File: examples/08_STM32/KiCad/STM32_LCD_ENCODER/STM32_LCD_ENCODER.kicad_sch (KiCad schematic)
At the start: 18 parts, among them J1 Audio In, SW1 ENCODER, U1 STM32F103C6Tx, U2 LCD16X2, X1 ACO-32.768MHz

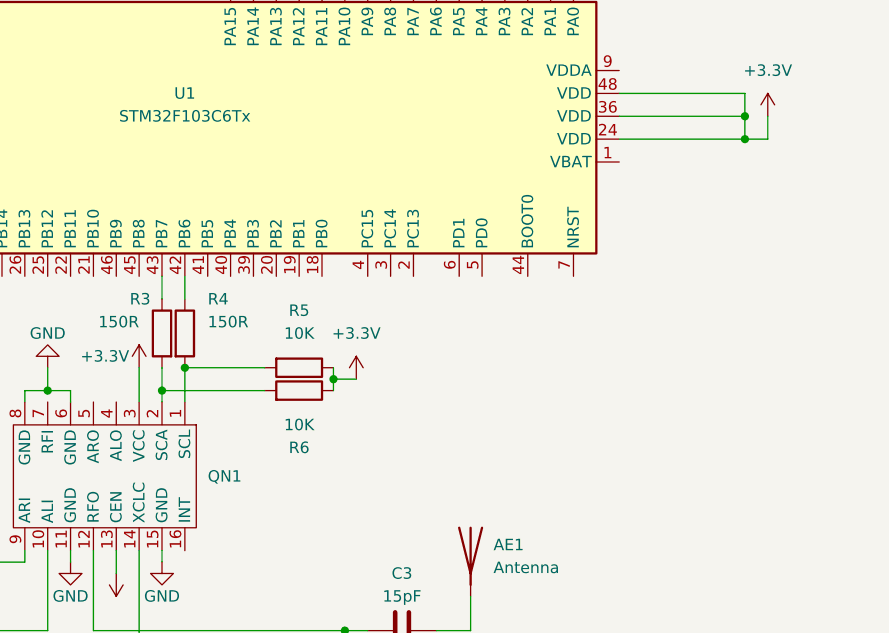
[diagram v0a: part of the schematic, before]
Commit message: Doc
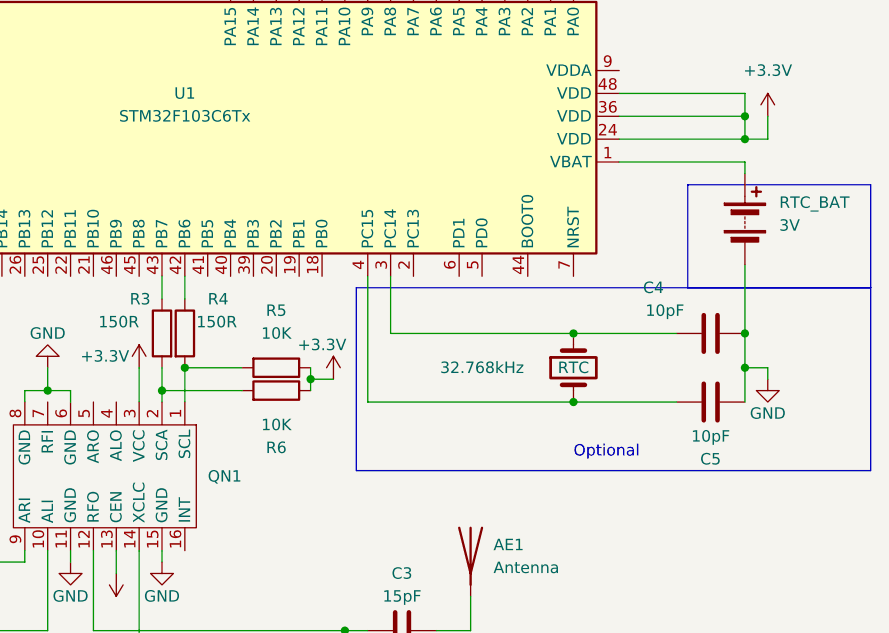
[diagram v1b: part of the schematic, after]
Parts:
- added C4, C5: 10pF, symbol Device:C
- added RTC: 32.768kHz, symbol Device:Crystal
- added RTC_BAT: 3V, symbol Device:Battery
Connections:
- net GND: now also C4.2, C5.2, RTC_BAT.2 (-)
- net at U1.1 (VBAT): now also RTC_BAT.1 (+)
- net at U1.3 (PC14): now also C4.1, RTC.1
- net at U1.4 (PC15): now also C5.1, RTC.2
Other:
- note added: "Optional"
- moved on the sheet: R5, R6
